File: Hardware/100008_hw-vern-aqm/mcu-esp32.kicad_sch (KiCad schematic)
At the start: 7 parts

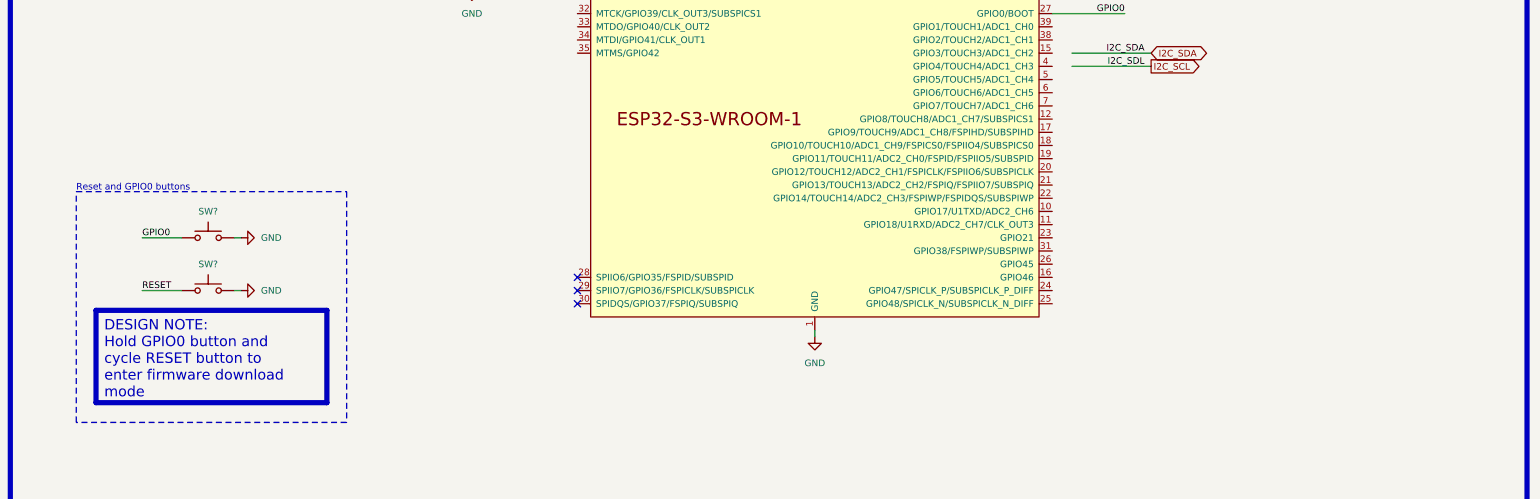
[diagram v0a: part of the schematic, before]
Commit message: schematic work
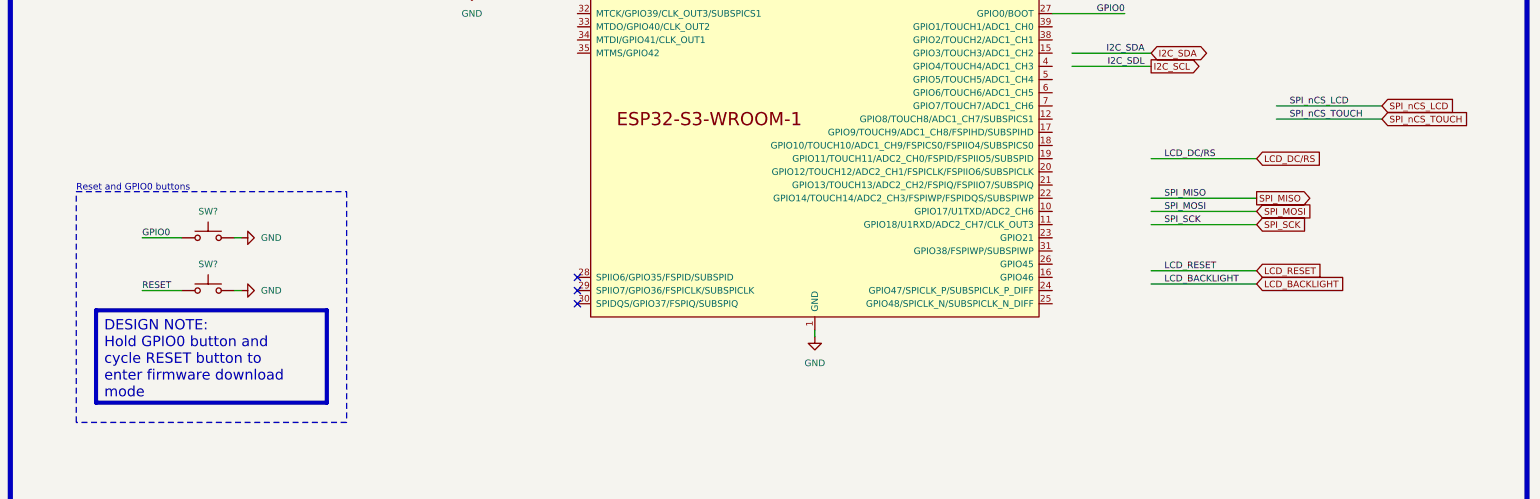
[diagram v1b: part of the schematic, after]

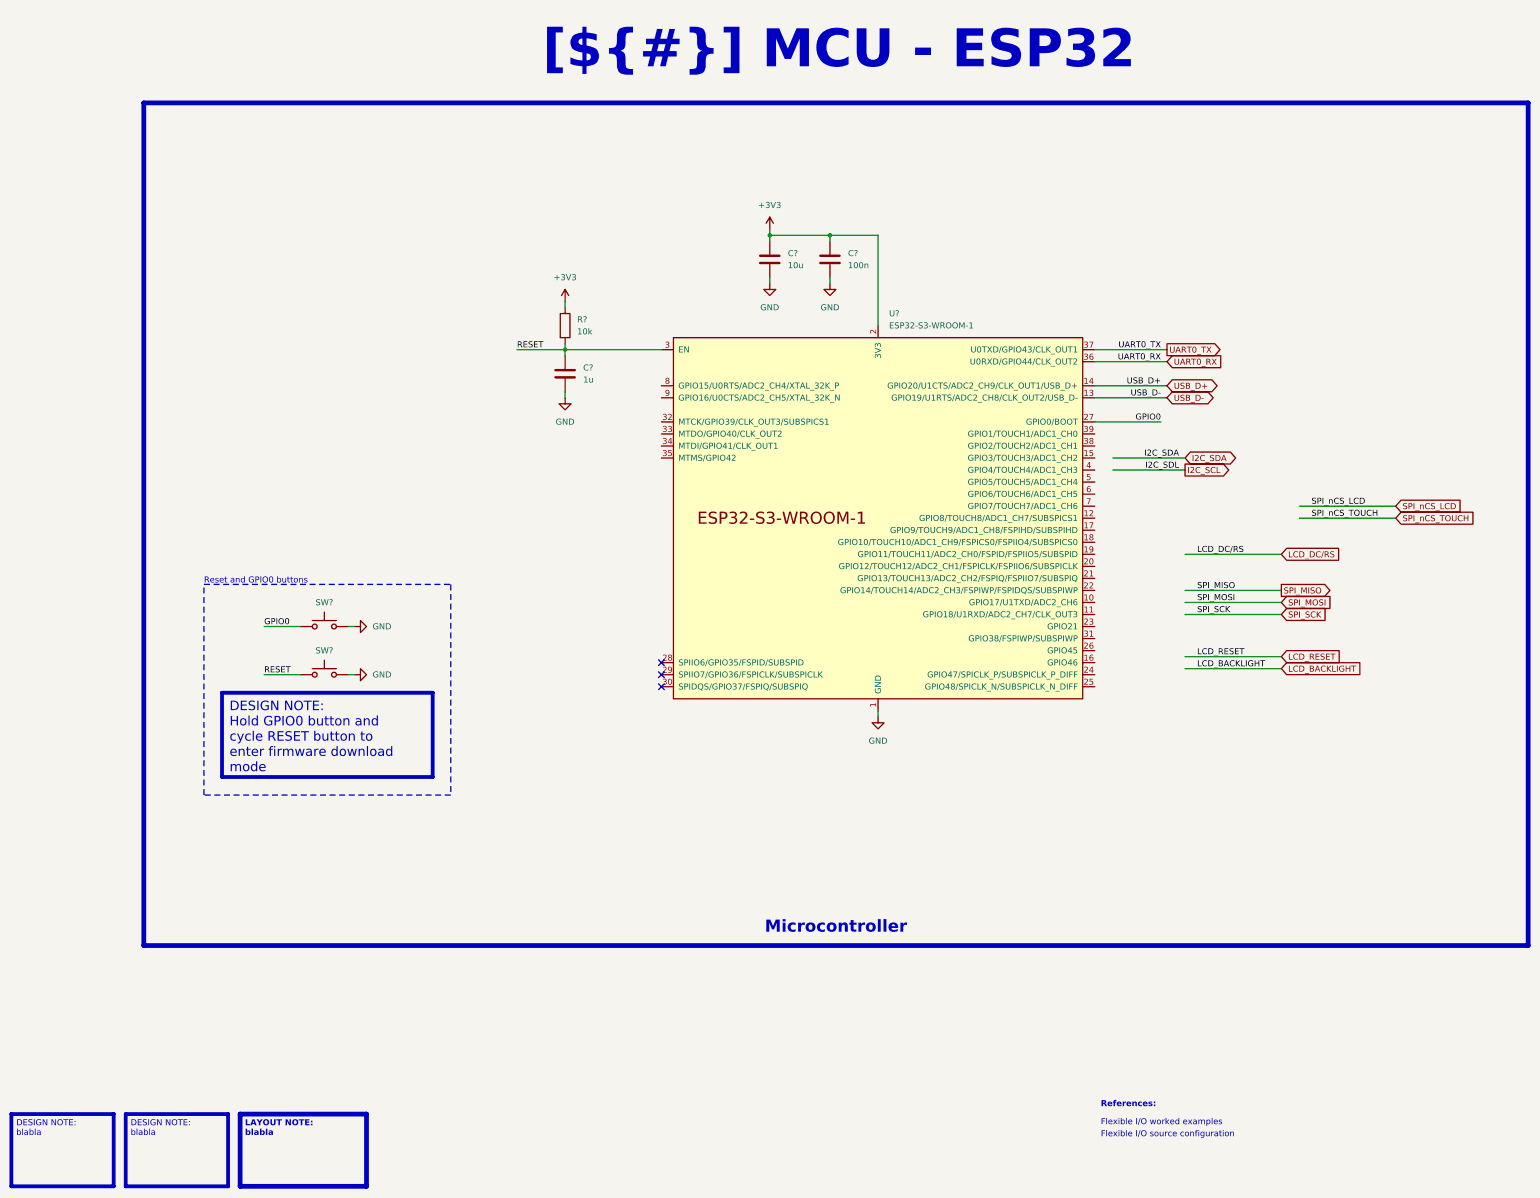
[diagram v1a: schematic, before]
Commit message: schematic work
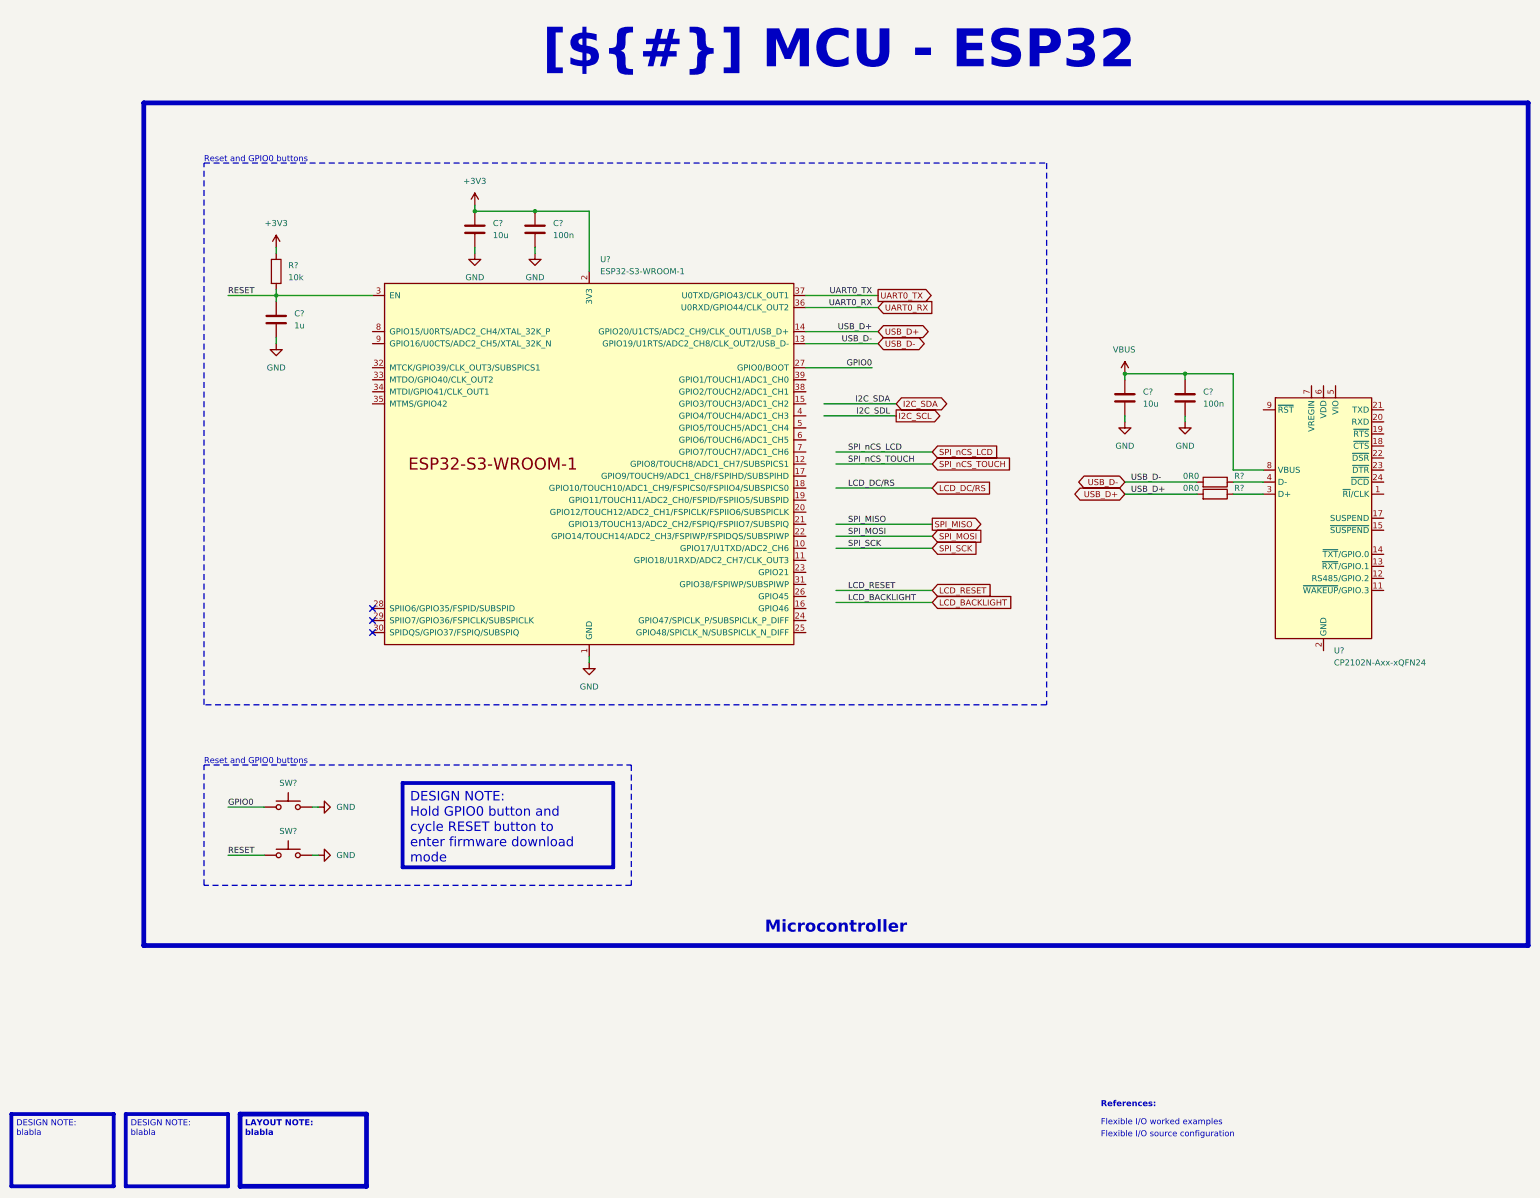
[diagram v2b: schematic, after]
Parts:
- added C?: 10u, Capacitor_SMD:C_0805_2012Metric, symbol Device:C
- added C?: 100n, Capacitor_SMD:C_0603_1608Metric, symbol Device:C
- added R? (x2): 0R0, Resistor_SMD:R_0603_1608Metric, symbol Device:R
- added U?: CP2102N-Axx-xQFN24, Package_DFN_QFN:QFN-24-1EP_4x4mm_P0.5mm_EP2.6x2.6mm, symbol Interface_USB:CP2102N-Axx-xQFN24
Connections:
- net GND: now also C?.2, C?.2
- net USB_D+: now also R?.2
- net USB_D-: now also R?.2
- new net: R?.1, U?.3 (D+)
- new net: R?.1, U?.4 (D-)
- new net: U?.2 (GND), U?.25 (GND)
- new net VBUS: C?.1, C?.1, U?.8 (VBUS)
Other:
- moved on the sheet: C?, R?, SW?, U?
